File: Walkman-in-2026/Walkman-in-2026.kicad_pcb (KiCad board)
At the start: 2 copper layers, 36 parts, among them J1 AudioJack3, J2 Micro_SD_Card, Q1 BSS138, Q2 BSS138, SW1 SW_Push, SW2 SW_Push, SW3 SW_Push, SW4 SW_SPST, SW5 SW_Push, SW6 SW_Push, U1 XIAO-ESP32-S3-DIP, U2 HS1602A-B, U3 PCM5102, U4 PCF8574P

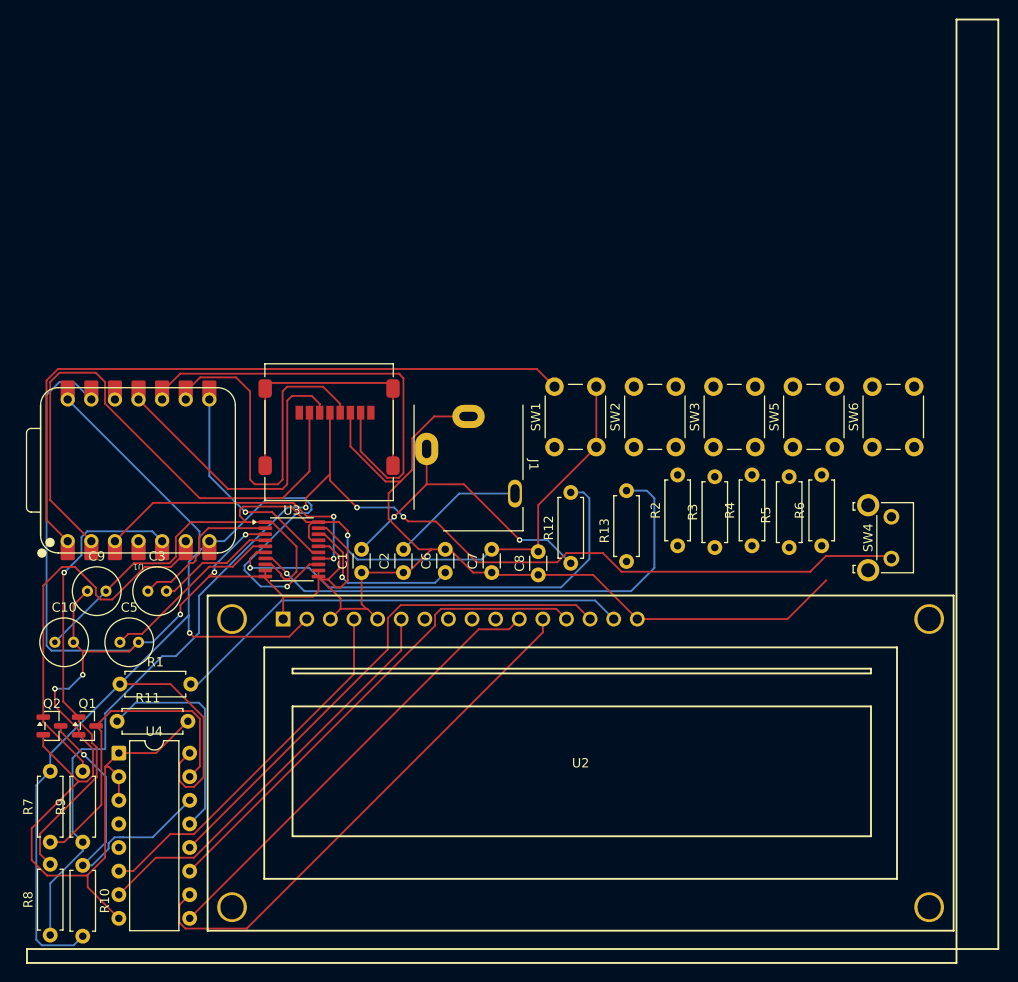
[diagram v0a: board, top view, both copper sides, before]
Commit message: may 6 session
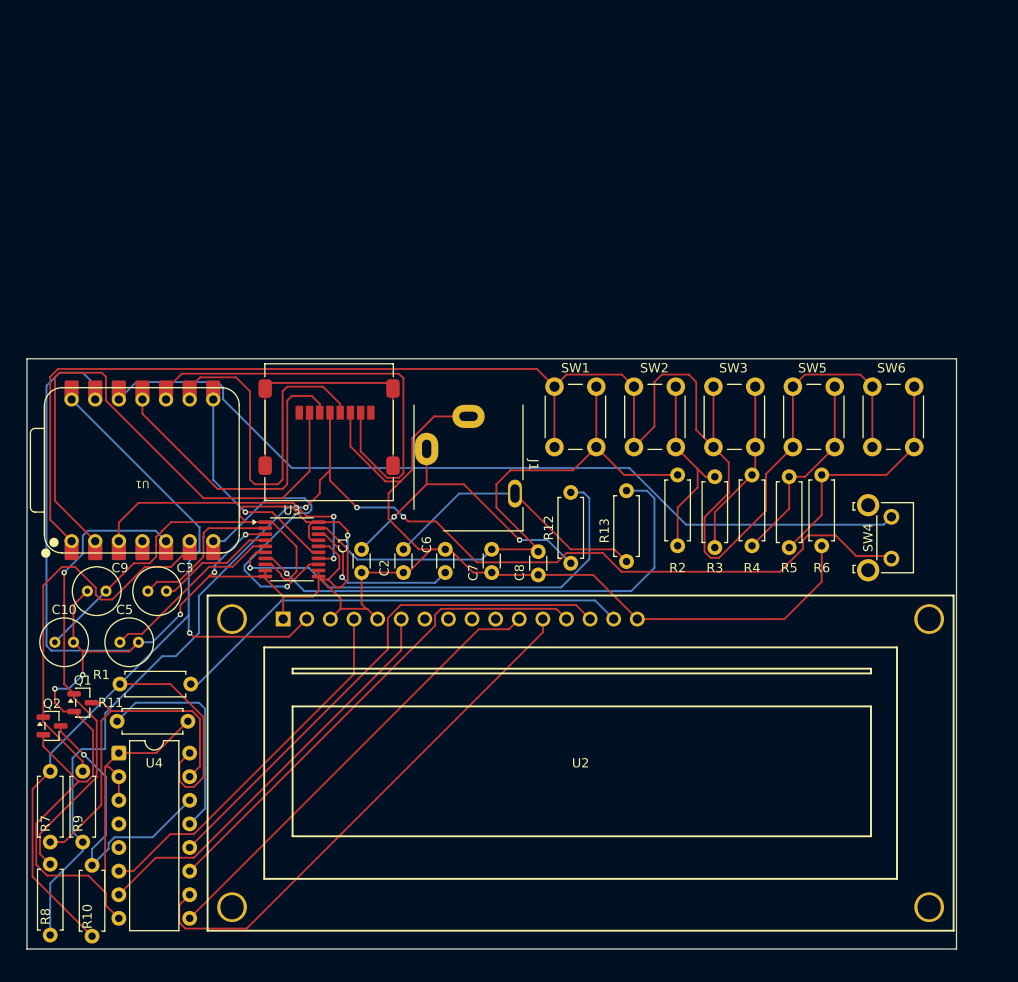
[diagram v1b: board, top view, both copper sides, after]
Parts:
- moved Q1 2.55 mm to (167.0, 110.5)
- moved R10 1.00 mm to (168.0, 128.0)
- moved U1 0.42 mm to (173.4, 85.5)
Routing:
- net Net-(U1-GPIO1_A0_D0): track 74.2 -> 176.7 mm
- net Net-(SW4-A): track 0.00 -> 91.3 mm
- net Net-(R5-Pad1): track 0.00 -> 27.0 mm
- net Net-(R4-Pad1): track 0.00 -> 21.8 mm
- net Net-(R2-Pad1): track 0.00 -> 21.2 mm
- net Net-(R3-Pad1): track 0.00 -> 19.1 mm
- net +3V3: track 102.8 -> 120.4 mm
- net Net-(C2-Pad2): track 14.5 -> 29.5 mm
- net GND: track 293.5 -> 300.8 mm
- net +5V: track 118.7 -> 112.7 mm
- net +3.3V: track 139.9 -> 142.7 mm
- net Net-(Q1-D): track 34.7 -> 36.7 mm
- net Net-(Q2-D): track 32.8 -> 31.4 mm
- net Net-(U1-GPIO3_A2_D2): track 32.3 -> 33.0 mm
- net Net-(J2-CLK): track 39.2 -> 39.9 mm
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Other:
- board outline added: 100 x 63.5 mm
